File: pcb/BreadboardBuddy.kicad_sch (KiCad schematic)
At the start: 0 parts

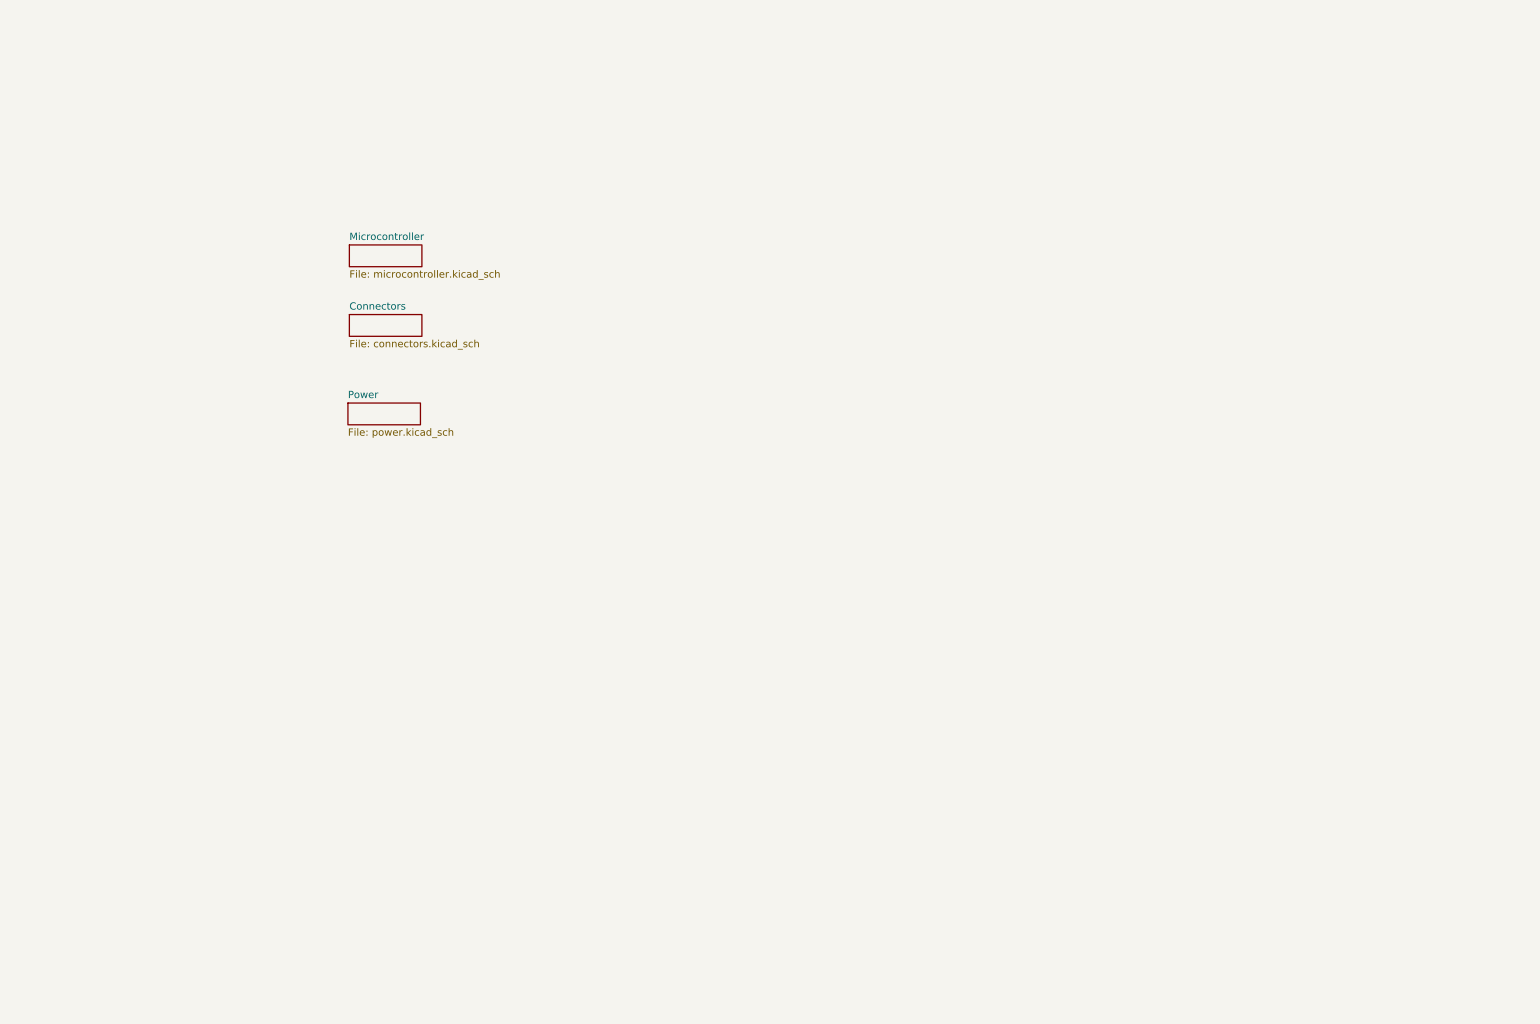
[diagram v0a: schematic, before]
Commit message: Prepped for DR
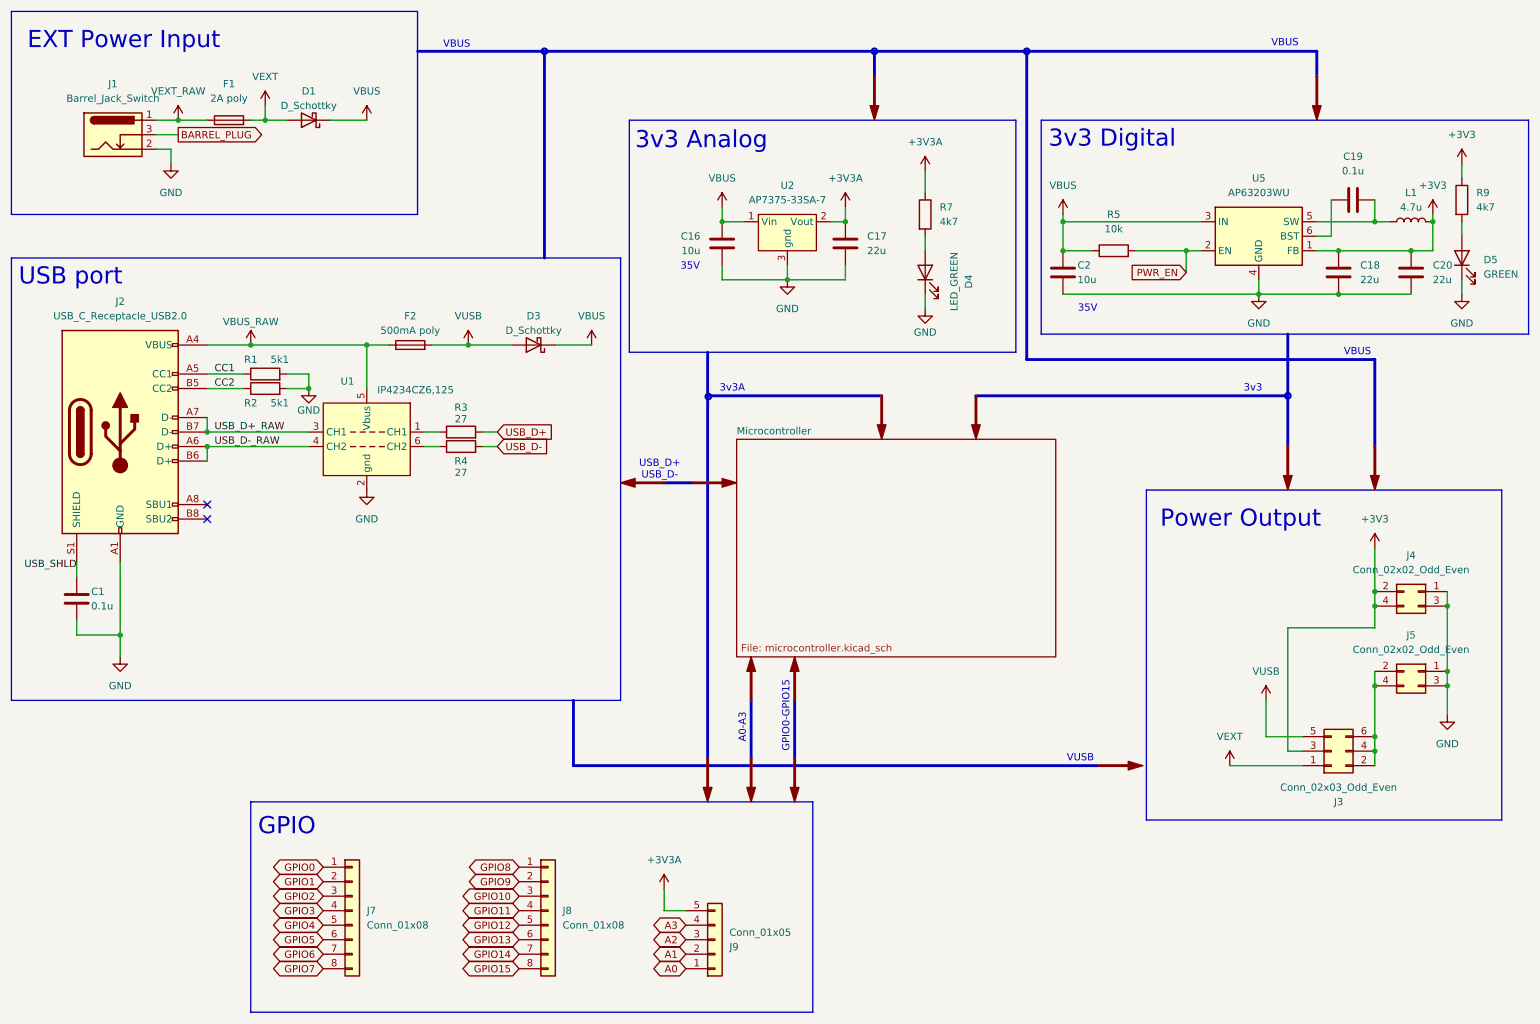
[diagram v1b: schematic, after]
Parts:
- added C1, C19: 0.1u, Capacitor_SMD:C_0603_1608Metric, symbol Device:C
- added C16, C2: 10u, Capacitor_SMD:C_0603_1608Metric, symbol Device:C
- added C17, C18, C20: 22u, Capacitor_SMD:C_0603_1608Metric, symbol Device:C
- added D1, D3: D_Schottky, Diode_SMD:D_1206_3216Metric, symbol Device:D_Schottky
- added D4: LED_GREEN, LED_SMD:LED_0603_1608Metric, symbol Device:LED
- added D5: GREEN, LED_SMD:LED_0603_1608Metric, symbol Device:LED
- added F1: 2A poly, Fuse:Fuse_1206_3216Metric, symbol Device:Fuse
- added F2: 500mA poly, Fuse:Fuse_1206_3216Metric, symbol Device:Fuse
- added J1: Barrel_Jack_Switch, Connector_BarrelJack:BarrelJack_Wuerth_6941xx301002, symbol Connector:Barrel_Jack_Switch
- added J2: USB_C_Receptacle_USB2.0, Connector_USB:USB_C_Receptacle_Palconn_UTC16-G, symbol Connector:USB_C_Receptacle_USB2.0
- added J3: Conn_02x03_Odd_Even, Connector_PinHeader_2.54mm:PinHeader_2x03_P2.54mm_Vertical, symbol Connector_Generic:Conn_02x03_Odd_Even
- added J4, J5: Conn_02x02_Odd_Even, Connector_PinHeader_2.54mm:PinHeader_2x02_P2.54mm_Vertical, symbol Connector_Generic:Conn_02x02_Odd_Even
- added J7, J8: Conn_01x08, Connector_PinHeader_2.54mm:PinHeader_1x08_P2.54mm_Vertical, symbol Connector_Generic:Conn_01x08
- added J9: Conn_01x05, Connector_PinHeader_2.54mm:PinHeader_1x05_P2.54mm_Vertical, symbol Connector_Generic:Conn_01x05
- added L1: 4.7u, Inductor_SMD:L_1210_3225Metric, symbol Device:L
- added R1, R2: 5k1, Resistor_SMD:R_0603_1608Metric, symbol Device:R
- added R3, R4: 27, Resistor_SMD:R_0603_1608Metric, symbol Device:R
- added R5: 10k, Resistor_SMD:R_0603_1608Metric, symbol Device:R
- added R7, R9: 4k7, Resistor_SMD:R_0603_1608Metric, symbol Device:R
- added U1: IP4234CZ6,125, Package_SO:TSOP-6_1.65x3.05mm_P0.95mm, symbol ip4234cz6:ip4234cz6
- added U2: AP7375-33SA-7, Package_TO_SOT_SMD:SOT-23, symbol BreadboardBuddy:AP7375_3.3v_linear_regulator
- added U5: AP63203WU, Package_TO_SOT_SMD:TSOT-23-6, symbol Regulator_Switching:AP63203WU
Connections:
- new net: D5.2 (A), R9.2
- new net: C19.2, L1.1, U5.5 (SW)
- new net: D4.2 (A), R7.2
- new net: R3.1, U1.1 (CH1)
- new net: C19.1, U5.6 (BST)
- new net: R4.1, U1.6 (CH2)
- new net: J3.2 (Pin_2), J3.4 (Pin_4), J3.6 (Pin_6), J5.2 (Pin_2), J5.4 (Pin_4)
- new net +3V3: C18.1, C20.1, J3.3 (Pin_3), J4.2 (Pin_2), J4.4 (Pin_4), L1.2, R9.1, U5.1 (FB)
- new net +3V3A: C17.1, J9.5 (Pin_5), R7.1, U2.2 (Vout)
- new net A0: J9.1 (Pin_1)
- new net A1: J9.2 (Pin_2)
- new net A2: J9.3 (Pin_3)
- new net A3: J9.4 (Pin_4)
- new net BARREL_PLUG: J1.3
- new net CC1: J2.A5 (CC1), R1.1
- new net CC2: J2.B5 (CC2), R2.1
- new net GND: C1.2, C16.2, C17.2, C18.2, C2.2, C20.2, D4.1 (K), D5.1 (K), J1.2, J2.A1 (GND), J2.A12 (GND), J2.B1 (GND), J2.B12 (GND), J4.1 (Pin_1), J4.3 (Pin_3), J5.1 (Pin_1), J5.3 (Pin_3), R1.2, R2.2, U1.2 (gnd), U2.3 (gnd), U5.4 (GND)
- new net GPIO0: J7.1 (Pin_1)
- new net GPIO1: J7.2 (Pin_2)
- new net GPIO10: J8.3 (Pin_3)
- new net GPIO11: J8.4 (Pin_4)
- new net GPIO12: J8.5 (Pin_5)
- new net GPIO13: J8.6 (Pin_6)
- new net GPIO14: J8.7 (Pin_7)
- new net GPIO15: J8.8 (Pin_8)
- new net GPIO2: J7.3 (Pin_3)
- new net GPIO3: J7.4 (Pin_4)
- new net GPIO4: J7.5 (Pin_5)
- new net GPIO5: J7.6 (Pin_6)
- new net GPIO6: J7.7 (Pin_7)
- new net GPIO7: J7.8 (Pin_8)
- new net GPIO8: J8.1 (Pin_1)
- new net GPIO9: J8.2 (Pin_2)
- new net PWR_EN: R5.2, U5.2 (EN)
- new net USB_D+: R3.2
- new net USB_D+_RAW: J2.A7 (D-), J2.B7 (D-), U1.3 (CH1)
- new net USB_D-: R4.2
- new net USB_D-_RAW: J2.A6 (D+), J2.B6 (D+), U1.4 (CH2)
- new net USB_SHLD: C1.1, J2.S1 (SHIELD)
- new net VBUS: C16.1, C2.1, D1.1 (K), D3.1 (K), R5.1, U2.1 (Vin), U5.3 (IN)
- new net VBUS_RAW: F2.1, J2.A4 (VBUS), J2.A9 (VBUS), J2.B4 (VBUS), J2.B9 (VBUS), U1.5 (Vbus)
- new net VEXT: D1.2 (A), F1.2, J3.1 (Pin_1)
- new net VEXT_RAW: F1.1, J1.1
- new net VUSB: D3.2 (A), F2.2, J3.5 (Pin_5)
- no-connect marks 0 -> 2
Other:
- removed sheet Connectors
- removed sheet Power
- note added: "35V"
- note added: "3v3"
- note added: "3v3 Analog"
- note added: "3v3 Digital"
- note added: "3v3A"
- note added: "A0-A3"
- note added: "EXT Power Input"
- note added: "GPIO"
- note added: "GPIO0-GPIO15"
- note added: "Power Output"
- note added: "USB port"
- note added: "USB_D+ USB_D-"
- note added: "VBUS"
- note added: "VUSB"
